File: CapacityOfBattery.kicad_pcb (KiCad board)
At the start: 2 copper layers, 30.5 x 57.1 mm, 21 parts, among them J1 BATTERY, J2 DUT, Q1 IRLML6401TRPBF, Q2 IRLML6401TRPBF, Q3 IRLML6401TRPBF, Q4 IRLML6401TRPBF, Q5 IRLML6401TRPBF

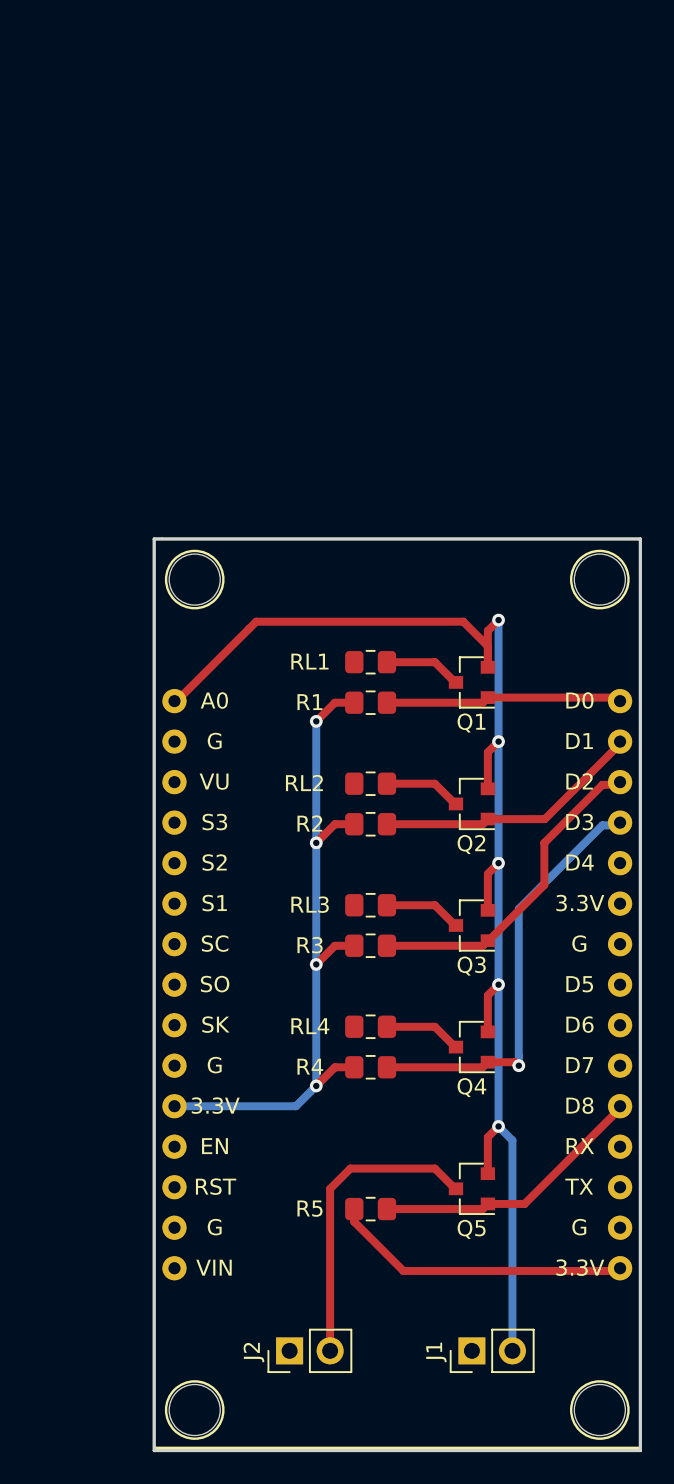
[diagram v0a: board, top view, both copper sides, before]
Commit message: updated pcb
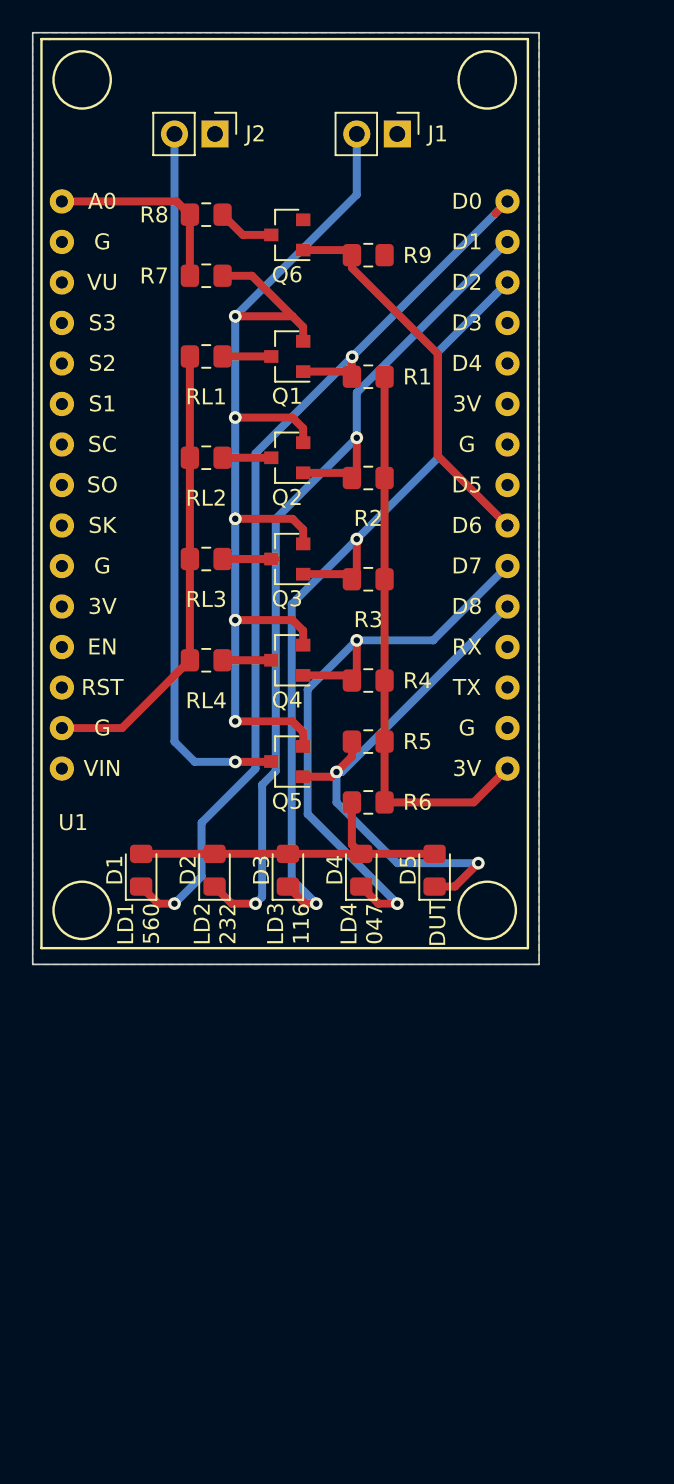
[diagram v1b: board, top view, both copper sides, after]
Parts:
- removed ?: For LOLin (NodeMCU v3), SUDHEENDRA_HEGDE:NodeMCU-LoLinV3
- removed ? (x4): MountingHole, MountingHole:MountingHole_3.2mm_M3
- added D1: LED, LED_SMD:LED_0805_2012Metric_Pad1.15x1.40mm_HandSolder, F.Cu at (19.5, 65.2)
- added D2: LED, LED_SMD:LED_0805_2012Metric_Pad1.15x1.40mm_HandSolder, F.Cu at (24.1, 65.2)
- added D3: LED, LED_SMD:LED_0805_2012Metric_Pad1.15x1.40mm_HandSolder, F.Cu at (28.7, 65.2)
- added D4: LED, LED_SMD:LED_0805_2012Metric_Pad1.15x1.40mm_HandSolder, F.Cu at (33.3, 65.2)
- added D5: LED, LED_SMD:LED_0805_2012Metric_Pad1.15x1.40mm_HandSolder, F.Cu at (37.9, 65.2)
- added Q6: SI2302, Package_TO_SOT_SMD:SOT-23, F.Cu at (28.7, 25.4)
- added R6: 560, Resistor_SMD:R_0805_2012Metric_Pad1.15x1.40mm_HandSolder, F.Cu at (33.7, 61.0)
- added R7: 60k, Resistor_SMD:R_0805_2012Metric_Pad1.15x1.40mm_HandSolder, F.Cu at (23.6, 27.9)
- added R8: 30k, Resistor_SMD:R_0805_2012Metric_Pad1.15x1.40mm_HandSolder, F.Cu at (23.6, 24.1)
- added R9: 10k, Resistor_SMD:R_0805_2012Metric_Pad1.15x1.40mm_HandSolder, F.Cu at (33.7, 26.6)
- added U1: NodeMCU1.0(ESP-12E), SUDHEENDRA_HEGDE:NodeMCU-LoLinV3, F.Cu at (28.5, 43.6)
- moved J1 76.4 mm to (35.6, 19.1), turned to 270 degrees
- moved J2 76.4 mm to (24.1, 19.1), turned to 270 degrees
- moved R5 29.3 mm to (33.7, 57.1), turned to 180 degrees
- moved Q5 29.2 mm to (28.7, 58.4)
- moved Q4 26.9 mm to (28.7, 52.0)
- moved Q3 25.7 mm to (28.7, 45.7)
- moved RL4 25.2 mm to (23.6, 52.0)
- moved Q2 24.6 mm to (28.7, 39.4)
- moved R4 24.3 mm to (33.7, 53.3), turned to 180 degrees
- moved RL3 24.0 mm to (23.6, 45.7)
- moved Q1 23.5 mm to (28.7, 33.0)
- moved R3 23.0 mm to (33.7, 47.0), turned to 180 degrees
- moved RL2 22.9 mm to (23.6, 39.4)
- moved RL1 21.8 mm to (23.6, 33.0)
- moved R2 21.7 mm to (33.7, 40.6), turned to 180 degrees
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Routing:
- net /Ctrl1: track 14.9 -> 60.7 mm, vias 0 -> 2
- net /Ctrl2: track 16.7 -> 56.9 mm, vias 0 -> 2
- net /Ctrl3: track 20.3 -> 53.3 mm, vias 0 -> 2
- net GND: track 0.00 -> 28.8 mm
- net /Vcc: track 62.5 -> 35.3 mm, vias 4 -> 0
- net Net-(J2-Pad2): track 19.1 -> 44.7 mm, vias 0 -> 1
- net /En_VoltageDivider: track 0.00 -> 24.2 mm
- net Net-(D1-Pad2): track 0.00 -> 21.9 mm
- net /Ctrl5: track 17.2 -> 35.5 mm, vias 0 -> 2
- net /Vbat: track 86.1 -> 72.6 mm
- net /Ctrl4: track 26.9 -> 40.0 mm, vias 1 -> 2
- net /Vin: track 0.00 -> 12.2 mm
- net Net-(Q6-Pad3): track 0.00 -> 3.58 mm
- net Net-(Q2-Pad3): track 4.85 -> 3.05 mm
- net Net-(Q4-Pad3): track 4.85 -> 3.05 mm
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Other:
- board size 30.5 x 57.1 mm -> 31.8 x 58.4 mm
- board text added: "DUT"
- board text added: "LD1 560"
- board text added: "LD2 232"
- board text added: "LD3 116"
- board text added: "LD4 047"

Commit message: updated pcb
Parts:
- RL2: value 330 -> 232
- RL3: value 100 -> 116
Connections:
- U1 pad 10: GND -> Net-(U1-Pad10)
- U1 pad 11: (no net) -> /Vcc
- U1 pad 17: GND -> Net-(U1-Pad17)
- U1 pad 2: GND -> Net-(U1-Pad2)
- U1 pad 24: GND -> Net-(U1-Pad24)
- U1 pad 25: (no net) -> Net-(U1-Pad25)
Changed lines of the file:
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@@
     (zones 0)
     (modules 27)
-    (nets 33)
+    (nets 38)
   )
   (page A4)
@@
   (net 31 "Net-(D1-Pad2)")
   (net 32 "Net-(J2-Pad2)")
+  (net 33 "Net-(U1-Pad25)")
+  (net 34 "Net-(U1-Pad24)")
+  (net 35 "Net-(U1-Pad17)")
+  (net 36 "Net-(U1-Pad10)")
+  (net 37 "Net-(U1-Pad2)")
   (net_class Default "This is the default net class."
     (clearance 0.5)
@@
     (add_net "Net-(Q4-Pad3)")
     (add_net "Net-(Q6-Pad3)")
+    (add_net "Net-(U1-Pad10)")
     (add_net "Net-(U1-Pad12)")
     (add_net "Net-(U1-Pad13)")
     (add_net "Net-(U1-Pad15)")
+    (add_net "Net-(U1-Pad17)")
     (add_net "Net-(U1-Pad18)")
     (add_net "Net-(U1-Pad19)")
+    (add_net "Net-(U1-Pad2)")
     (add_net "Net-(U1-Pad23)")
+    (add_net "Net-(U1-Pad24)")
+    (add_net "Net-(U1-Pad25)")
     (add_net "Net-(U1-Pad26)")
     (add_net "Net-(U1-Pad27)")
@@
     (pad 26 thru_hole circle (at 13.97 -10.16) (size 1.524 1.524) (drill 0.762) (layers *.Cu *.Mask F.SilkS)
       (net 5 "Net-(U1-Pad26)"))
-    (pad 25 thru_hole circle (at 13.97 -7.62) (size 1.524 1.524) (drill 0.762) (layers *.Cu *.Mask F.SilkS))
+    (pad 25 thru_hole circle (at 13.97 -7.62) (size 1.524 1.524) (drill 0.762) (layers *.Cu *.Mask F.SilkS)
+      (net 33 "Net-(U1-Pad25)"))
     (pad 24 thru_hole circle (at 13.97 -5.08) (size 1.524 1.524) (drill 0.762) (layers *.Cu *.Mask F.SilkS)
-      (net 11 GND))
+      (net 34 "Net-(U1-Pad24)"))
     (pad 23 thru_hole circle (at 13.97 -2.54) (size 1.524 1.524) (drill 0.762) (layers *.Cu *.Mask F.SilkS)
       (net 6 "Net-(U1-Pad23)"))
@@
       (net 9 "Net-(U1-Pad18)"))
     (pad 17 thru_hole circle (at 13.97 12.7) (size 1.524 1.524) (drill 0.762) (layers *.Cu *.Mask F.SilkS)
-      (net 11 GND))
+      (net 35 "Net-(U1-Pad17)"))
     (pad 16 thru_hole circle (at 13.97 15.24) (size 1.524 1.524) (drill 0.762) (layers *.Cu *.Mask F.SilkS)
       (net 14 /Vcc))
@@
     (pad 12 thru_hole circle (at -13.97 7.62) (size 1.524 1.524) (drill 0.762) (layers *.Cu *.Mask F.SilkS)
       (net 13 "Net-(U1-Pad12)"))
-    (pad 11 thru_hole circle (at -13.97 5.08) (size 1.524 1.524) (drill 0.762) (layers *.Cu *.Mask F.SilkS))
+    (pad 11 thru_hole circle (at -13.97 5.08) (size 1.524 1.524) (drill 0.762) (layers *.Cu *.Mask F.SilkS)
+      (net 14 /Vcc))
     (pad 10 thru_hole circle (at -13.97 2.54) (size 1.524 1.524) (drill 0.762) (layers *.Cu *.Mask F.SilkS)
-      (net 11 GND))
+      (net 36 "Net-(U1-Pad10)"))
     (pad 9 thru_hole circle (at -13.97 0) (size 1.524 1.524) (drill 0.762) (layers *.Cu *.Mask F.SilkS)
       (net 15 "Net-(U1-Pad9)"))
@@
       (net 21 "Net-(U1-Pad3)"))
     (pad 2 thru_hole circle (at -13.97 -17.78) (size 1.524 1.524) (drill 0.762) (layers *.Cu *.Mask F.SilkS)
-      (net 11 GND))
+      (net 37 "Net-(U1-Pad2)"))
     (pad 1 thru_hole circle (at -13.97 -20.32) (size 1.524 1.524) (drill 0.762) (layers *.Cu *.Mask F.SilkS)
       (net 29 /Vin))
@@
       (effects (font (size 1 1) (thickness 0.15)))
     )
-    (fp_text value 330 (at 0 1.65) (layer F.Fab)
+    (fp_text value 232 (at 0 1.65) (layer F.Fab)
       (effects (font (size 1 1) (thickness 0.15)))
     )
@@
       (effects (font (size 1 1) (thickness 0.15)))
     )
-    (fp_text value 100 (at 0 1.65) (layer F.Fab)
+    (fp_text value 116 (at 0 1.65) (layer F.Fab)
       (effects (font (size 1 1) (thickness 0.15)))
     )
@@
     (effects (font (size 1 1) (thickness 0.15)))
   )
-  (via (at 31.75 59.055) (size 0.8) (drill 0.4) (layers F.Cu B.Cu) (net 7))
   (via (at 21.59 67.31) (size 0.8) (drill 0.4) (layers F.Cu B.Cu) (net 1))
-  (via (at 26.67 67.31) (size 0.8) (drill 0.4) (layers F.Cu B.Cu) (net 2))
-  (via (at 30.48 67.31) (size 0.8) (drill 0.4) (layers F.Cu B.Cu) (net 3))
-  (via (at 40.64 64.77) (size 0.8) (drill 0.4) (layers F.Cu B.Cu) (net 7))
-  (via (at 35.56 67.31) (size 0.8) (drill 0.4) (layers F.Cu B.Cu) (net 4))
-  (via (at 25.4 58.42) (size 0.8) (drill 0.4) (layers F.Cu B.Cu) (net 32))
-  (via (at 33.02 38.1) (size 0.8) (drill 0.4) (layers F.Cu B.Cu) (net 2))
-  (via (at 33.02 44.45) (size 0.8) (drill 0.4) (layers F.Cu B.Cu) (net 3))
-  (via (at 33.02 50.8) (size 0.8) (drill 0.4) (layers F.Cu B.Cu) (net 4))
   (segment (start 32.395 33.95) (end 32.715 34.27) (width 0.5) (layer F.Cu) (net 1))
   (segment (start 29.66 33.95) (end 32.395 33.95) (width 0.5) (layer F.Cu) (net 1))
@@
   (segment (start 32.715 33.035) (end 32.73 33.02) (width 0.5) (layer F.Cu) (net 1))
   (segment (start 32.715 34.27) (end 32.715 33.035) (width 0.5) (layer F.Cu) (net 1))
+  (via (at 26.67 67.31) (size 0.8) (drill 0.4) (layers F.Cu B.Cu) (net 2))
+  (via (at 33.02 38.1) (size 0.8) (drill 0.4) (layers F.Cu B.Cu) (net 2))
   (segment (start 32.395 40.3) (end 32.715 40.62) (width 0.5) (layer F.Cu) (net 2))
   (segment (start 29.66 40.3) (end 32.395 40.3) (width 0.5) (layer F.Cu) (net 2))
@@
   (segment (start 25.175899 67.31) (end 24.100833 66.234934) (width 0.5) (layer F.Cu) (net 2))
   (segment (start 26.67 67.31) (end 25.175899 67.31) (width 0.5) (layer F.Cu) (net 2))
+  (via (at 30.48 67.31) (size 0.8) (drill 0.4) (layers F.Cu B.Cu) (net 3))
+  (via (at 33.02 44.45) (size 0.8) (drill 0.4) (layers F.Cu B.Cu) (net 3))
   (segment (start 32.395 46.65) (end 32.715 46.97) (width 0.5) (layer F.Cu) (net 3))
   (segment (start 29.66 46.65) (end 32.395 46.65) (width 0.5) (layer F.Cu) (net 3))
@@
   (segment (start 29.775899 67.31) (end 28.700833 66.234934) (width 0.5) (layer F.Cu) (net 3))
   (segment (start 30.48 67.31) (end 29.775899 67.31) (width 0.5) (layer F.Cu) (net 3))
+  (via (at 35.56 67.31) (size 0.8) (drill 0.4) (layers F.Cu B.Cu) (net 4))
+  (via (at 33.02 50.8) (size 0.8) (drill 0.4) (layers F.Cu B.Cu) (net 4))
   (segment (start 32.395 53) (end 32.715 53.32) (width 0.5) (layer F.Cu) (net 4))
   (segment (start 29.66 53) (end 32.395 53) (width 0.5) (layer F.Cu) (net 4))
@@
   (segment (start 34.375899 67.31) (end 33.300833 66.234934) (width 0.5) (layer F.Cu) (net 4))
   (segment (start 35.56 67.31) (end 34.375899 67.31) (width 0.5) (layer F.Cu) (net 4))
+  (via (at 31.75 59.055) (size 0.8) (drill 0.4) (layers F.Cu B.Cu) (net 7))
+  (via (at 40.64 64.77) (size 0.8) (drill 0.4) (layers F.Cu B.Cu) (net 7))
   (segment (start 42.47 48.97) (end 42.47 48.68) (width 0.5) (layer B.Cu) (net 7))
   (segment (start 39.175066 66.234934) (end 37.900833 66.234934) (width 0.5) (layer F.Cu) (net 7))
@@
   (segment (start 22.555 33) (end 22.555 39.35) (width 0.5) (layer F.Cu) (net 11))
   (segment (start 22.555 39.35) (end 22.555 45.7) (width 0.5) (layer F.Cu) (net 11))
-  (via (at 25.4 30.48) (size 0.8) (drill 0.4) (layers F.Cu B.Cu) (net 22))
-  (via (at 25.4 36.83) (size 0.8) (drill 0.4) (layers F.Cu B.Cu) (net 22))
-  (via (at 25.4 43.18) (size 0.8) (drill 0.4) (layers F.Cu B.Cu) (net 22))
-  (via (at 25.4 49.53) (size 0.8) (drill 0.4) (layers F.Cu B.Cu) (net 22))
-  (via (at 25.4 55.88) (size 0.8) (drill 0.4) (layers F.Cu B.Cu) (net 22))
   (segment (start 34.765 57.15) (end 34.765 60.96) (width 0.5) (layer F.Cu) (net 14))
   (segment (start 40.35 60.96) (end 42.47 58.84) (width 0.5) (layer F.Cu) (net 14))
@@
   (segment (start 34.765 34.27) (end 34.765 40.62) (width 0.5) (layer F.Cu) (net 14))
   (segment (start 34.765 57.15) (end 34.765 53.32) (width 0.5) (layer F.Cu) (net 14))
+  (via (at 25.4 30.48) (size 0.8) (drill 0.4) (layers F.Cu B.Cu) (net 22))
+  (via (at 25.4 36.83) (size 0.8) (drill 0.4) (layers F.Cu B.Cu) (net 22))
+  (via (at 25.4 43.18) (size 0.8) (drill 0.4) (layers F.Cu B.Cu) (net 22))
+  (via (at 25.4 49.53) (size 0.8) (drill 0.4) (layers F.Cu B.Cu) (net 22))
+  (via (at 25.4 55.88) (size 0.8) (drill 0.4) (layers F.Cu B.Cu) (net 22))
   (segment (start 29.66 31.15) (end 29.66 32.05) (width 0.5) (layer F.Cu) (net 22))
   (segment (start 24.605 27.94) (end 26.45 27.94) (width 0.5) (layer F.Cu) (net 22))
@@
   (segment (start 19.500833 64.184934) (end 24.100833 64.184934) (width 0.5) (layer F.Cu) (net 31))
   (segment (start 24.100833 64.184934) (end 28.700833 64.184934) (width 0.5) (layer F.Cu) (net 31))
+  (via (at 25.4 58.42) (size 0.8) (drill 0.4) (layers F.Cu B.Cu) (net 32))
   (segment (start 27.64 58.42) (end 27.66 58.4) (width 0.5) (layer F.Cu) (net 32))
   (segment (start 25.4 58.42) (end 27.64 58.42) (width 0.5) (layer F.Cu) (net 32))
